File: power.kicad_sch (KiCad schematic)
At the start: 11 parts, among them J2 USB_C_Receptacle_USB2.0_16P, J3 BATTERY, U5 LD1117S33TR_SOT223

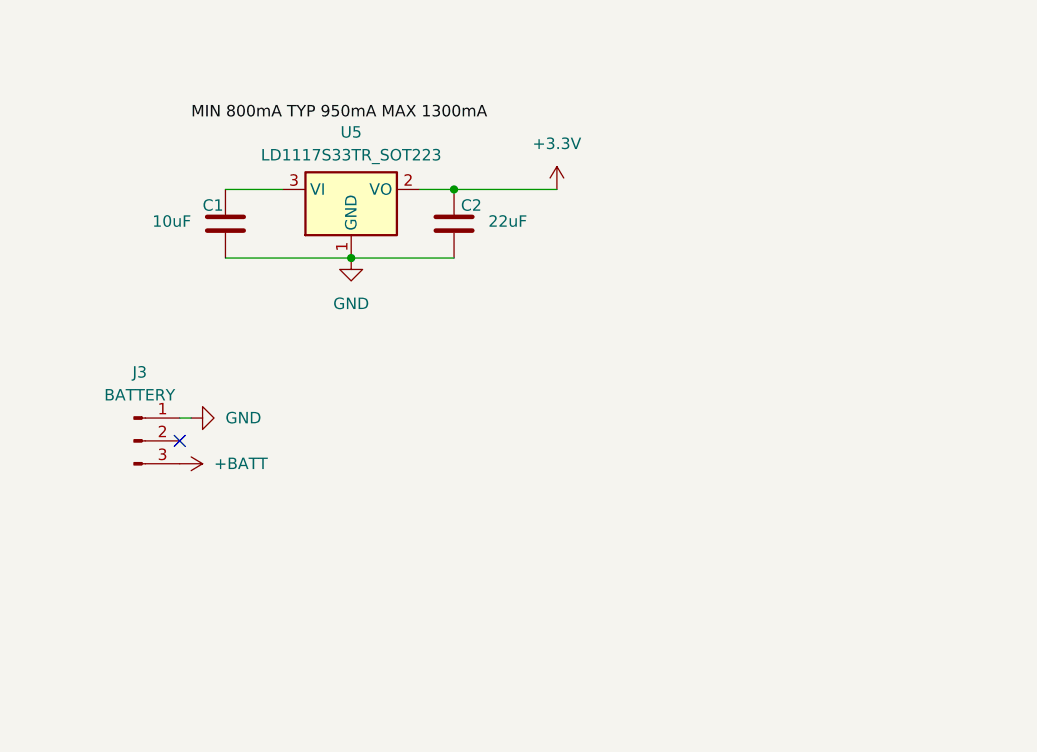
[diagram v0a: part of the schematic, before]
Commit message: power
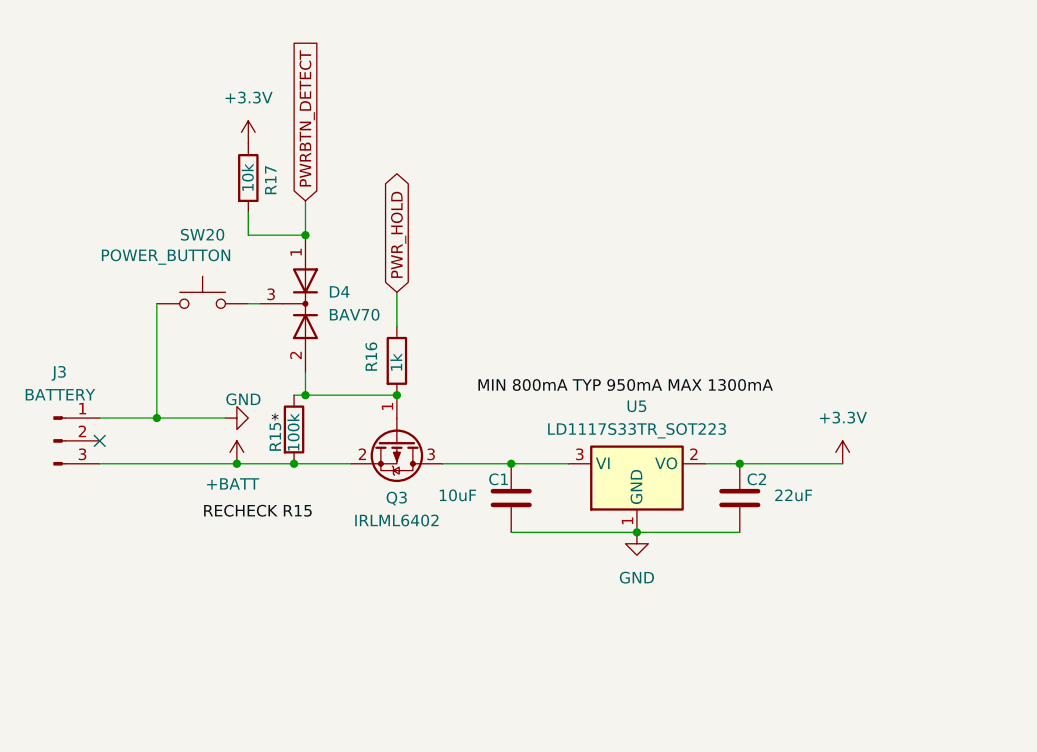
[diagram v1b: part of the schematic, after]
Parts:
- added D4: BAV70, Package_TO_SOT_SMD:SOT-23, symbol Diode:BAV70
- added Q3: IRLML6402, Package_TO_SOT_SMD:SOT-23, symbol Transistor_FET:IRLML6402
- added R15: 100k, symbol Device:R
- added R16: 1k, symbol Device:R
- added R17: 10k, symbol Device:R
- added SW20: POWER_BUTTON, symbol Switch:SW_Push
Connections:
- net +3.3V: now also R17.1
- net +BATT: now also Q3.2 (S), R15.2
- net GND: now also SW20.1
- net at C1.1, U5.3 (VI): now also Q3.3 (D)
- new net: D4.2 (A), Q3.1 (G), R15.1, R16.2
- new net: D4.3 (K), SW20.2
- new net PWRBTN_DETECT: D4.1 (A), R17.2
- new net PWR_HOLD: R16.1
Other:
- moved on the sheet: C1, C2, J3, U5

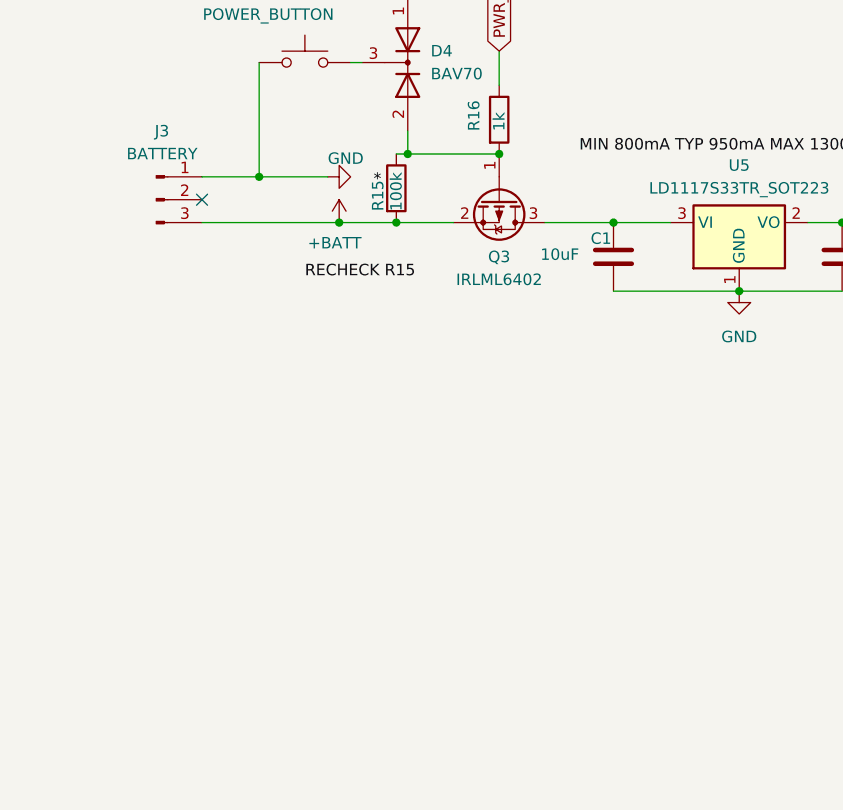
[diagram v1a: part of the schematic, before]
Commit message: spi joke
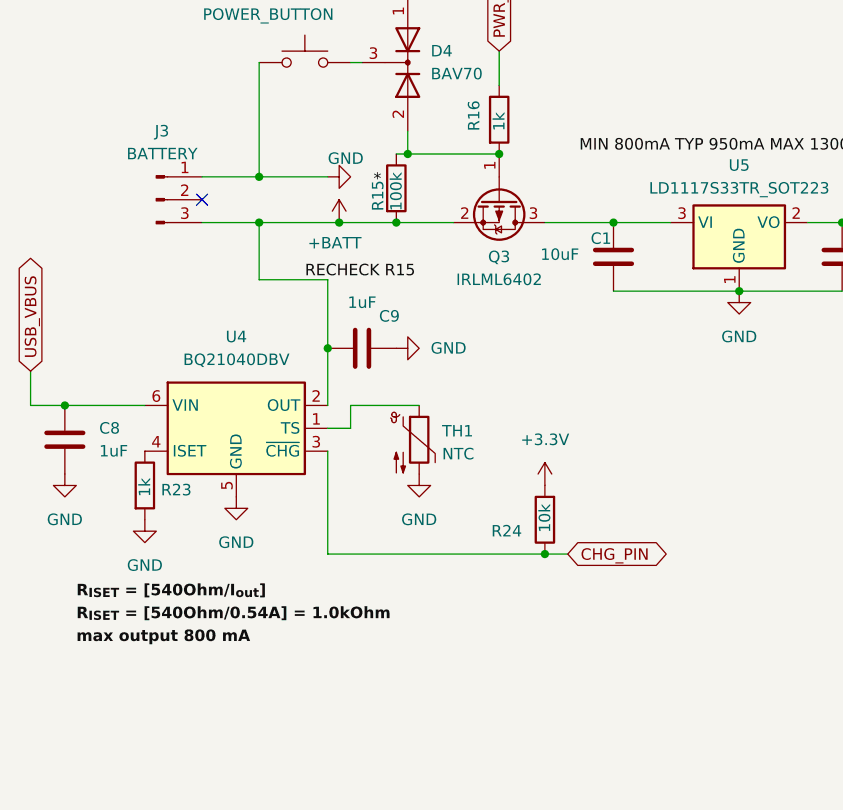
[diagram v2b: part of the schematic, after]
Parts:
- added C8, C9: 1uF, symbol Device:C
- added R23: 1k, symbol Device:R
- added R24: 10k, symbol Device:R
- added TH1: NTC, symbol Device:Thermistor_NTC
- added U4: BQ21040DBV, Package_TO_SOT_SMD:SOT-23-6, symbol Battery_Management:BQ21040DBV
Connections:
- net +3.3V: now also R24.2
- net +BATT: now also C9.1, U4.2 (OUT)
- net GND: now also C8.2, C9.2, R23.2, TH1.2, U4.5 (GND)
- net USB_VBUS: now also C8.1, U4.6 (VIN)
- new net: R23.1, U4.4 (ISET)
- new net: TH1.1, U4.1 (TS)
- new net CHG_PIN: R24.1, U4.3 (~{CHG})

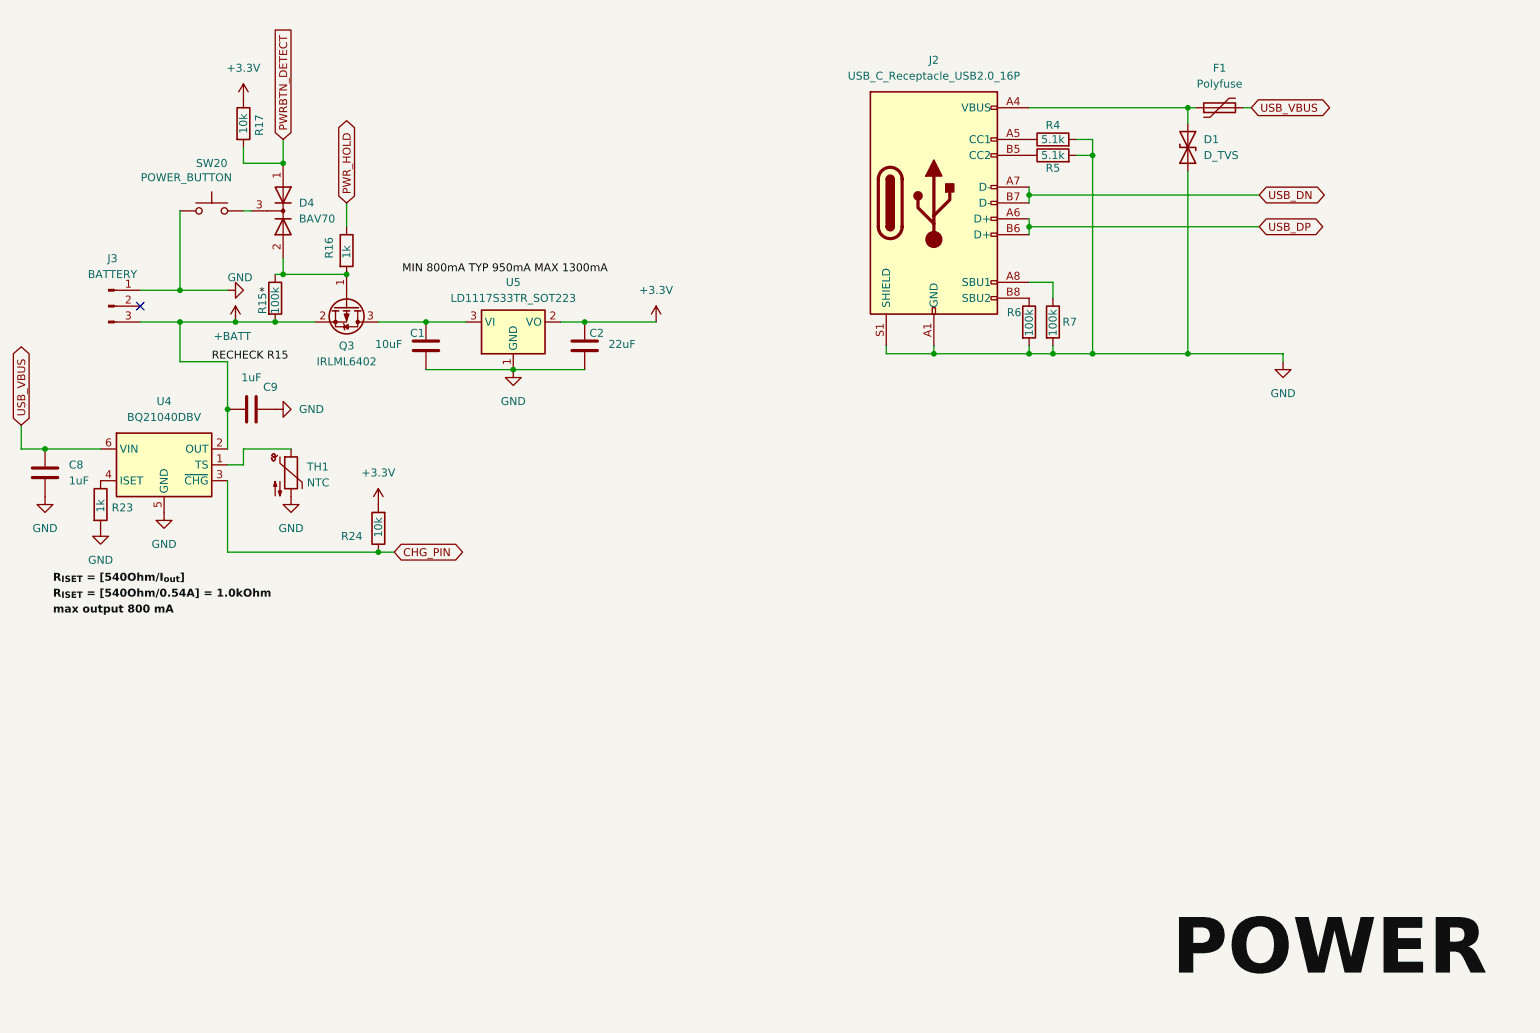
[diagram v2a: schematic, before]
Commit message: buck converter
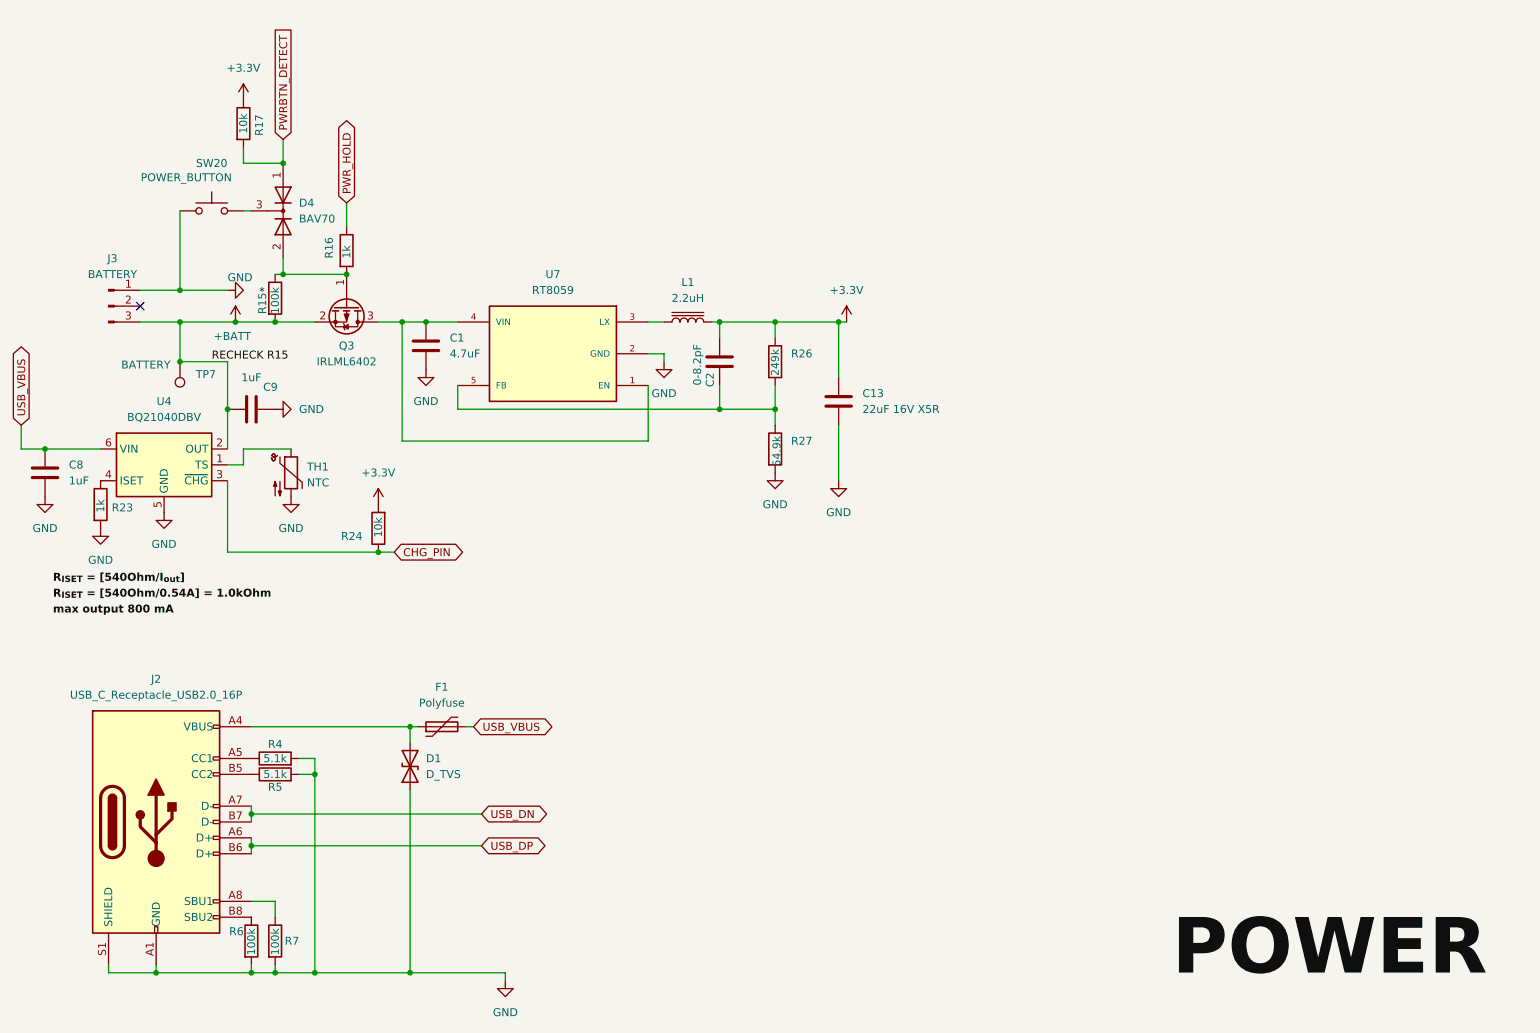
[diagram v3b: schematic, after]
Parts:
- removed U5: LD1117S33TR_SOT223, Package_TO_SOT_SMD:SOT-223-3_TabPin2, symbol Regulator_Linear:LD1117S33TR_SOT223
- added C13: 22uF 16V X5R, Capacitor_SMD:C_1206_3216Metric, symbol Device:C
- added L1: 2.2uH, Inductor_SMD:L_6.3x6.3_H3, symbol Device:L_Iron
- added R26: 249k, symbol Device:R
- added R27: 54.9k, symbol Device:R
- added TP7: BATTERY, symbol Connector:TestPoint
- added U7: RT8059, Package_TO_SOT_SMD:TSOT-23-5_HandSoldering, symbol RT8059:RT8059
- C1: value 10uF -> 4.7uF; footprint (none) -> Capacitor_SMD:C_0603_1608Metric
- C2: value 22uF -> 0-8.2pF; footprint (none) -> Capacitor_SMD:C_0603_1608Metric_Pad1.08x0.95mm_HandSolder
- R4: footprint (none) -> Capacitor_SMD:C_0603_1608Metric_Pad1.08x0.95mm_HandSolder
- TH1: footprint (none) -> Connector_JST:JST_EH_B2B-EH-A_1x02_P2.50mm_Vertical
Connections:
- net +3.3V: now also C13.1, L1.2, R26.1
- net +BATT: now also TP7.1
- net GND: now also C13.2, R27.2, U7.2 (GND); no longer C2.2
- net at C1.1, Q3.3 (D): now also U7.1 (EN), U7.4 (VIN)
- new net: C2.2, R26.2, R27.1, U7.5 (FB)
- new net: L1.1, U7.3 (LX)
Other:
- moved on the sheet: D1, F1, J2, R4, R5, R6, R7
